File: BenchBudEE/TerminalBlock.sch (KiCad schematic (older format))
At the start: 0 parts

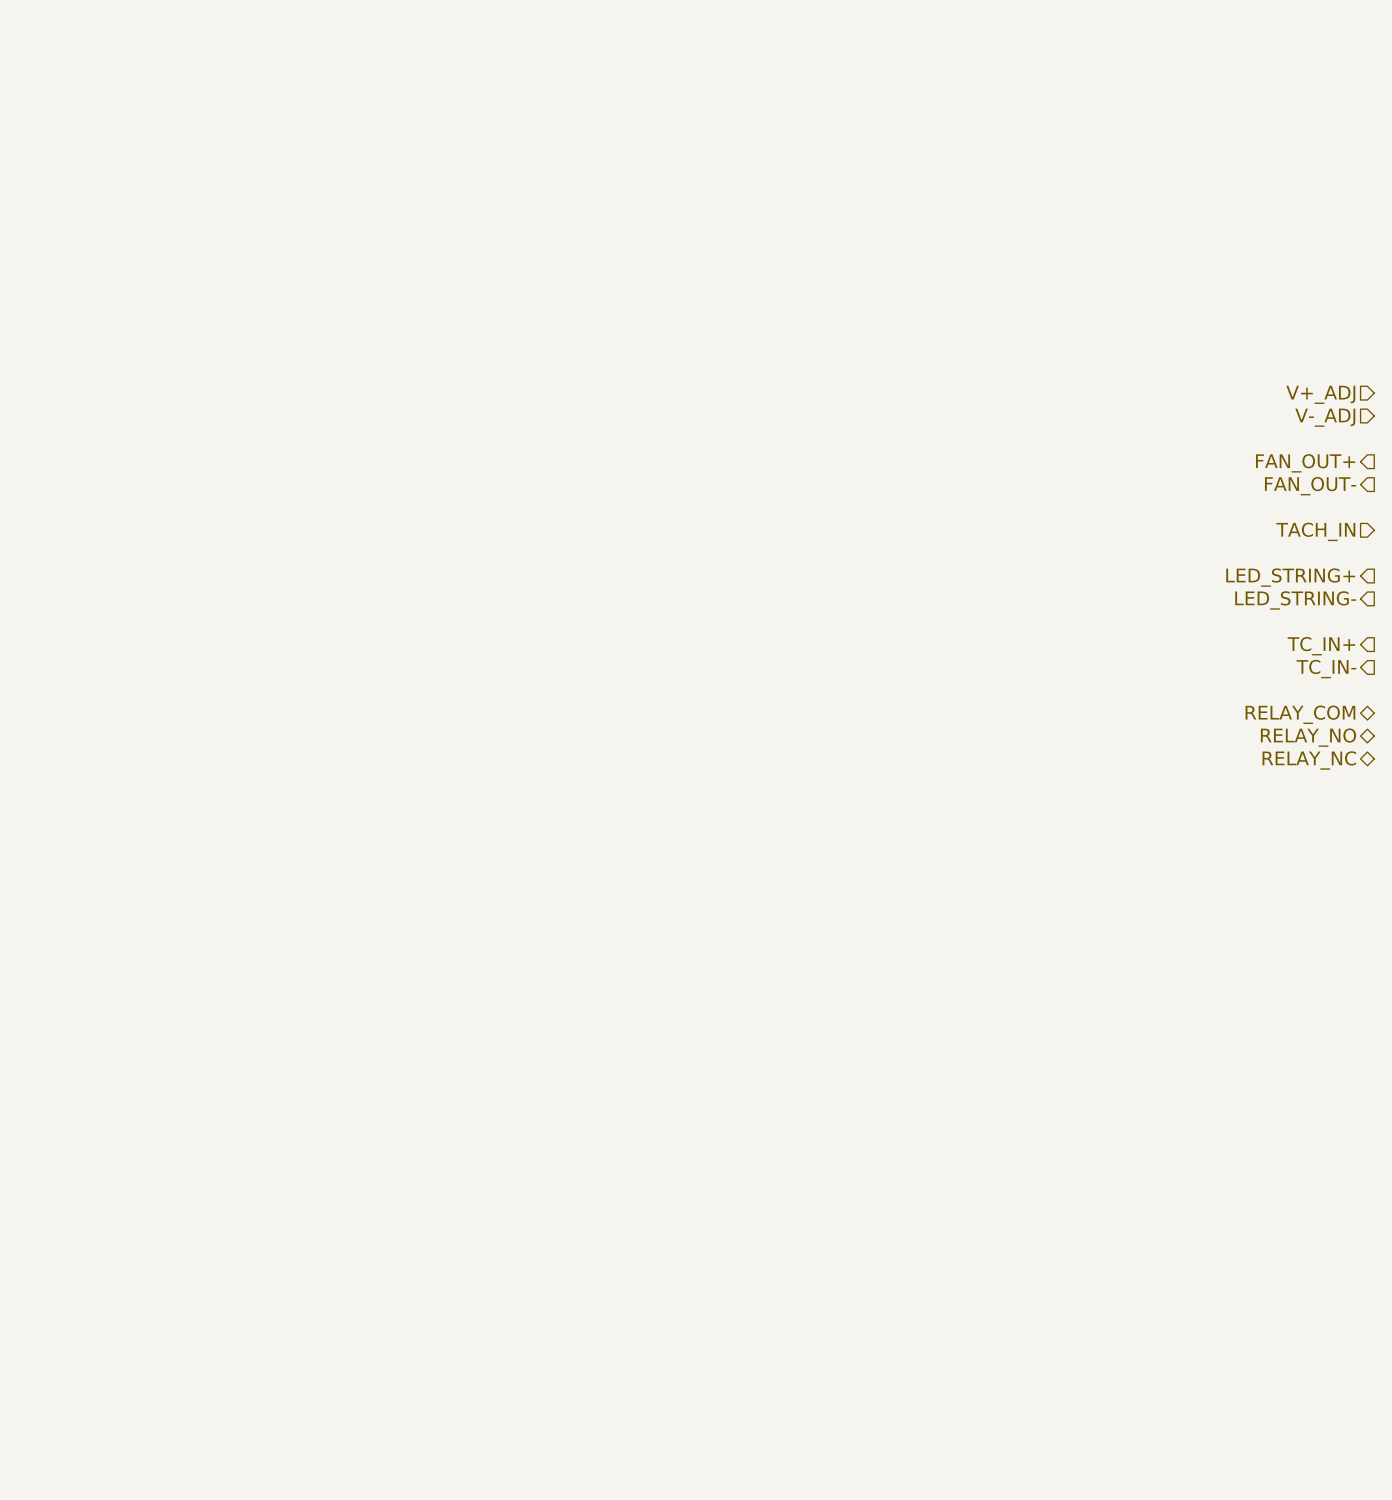
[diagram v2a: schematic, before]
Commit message: syncing to https://github.com/ContextualElectronics/BenchBudEE/tree/ebd662c68b928f78643cdf924dc35a4d91f03121
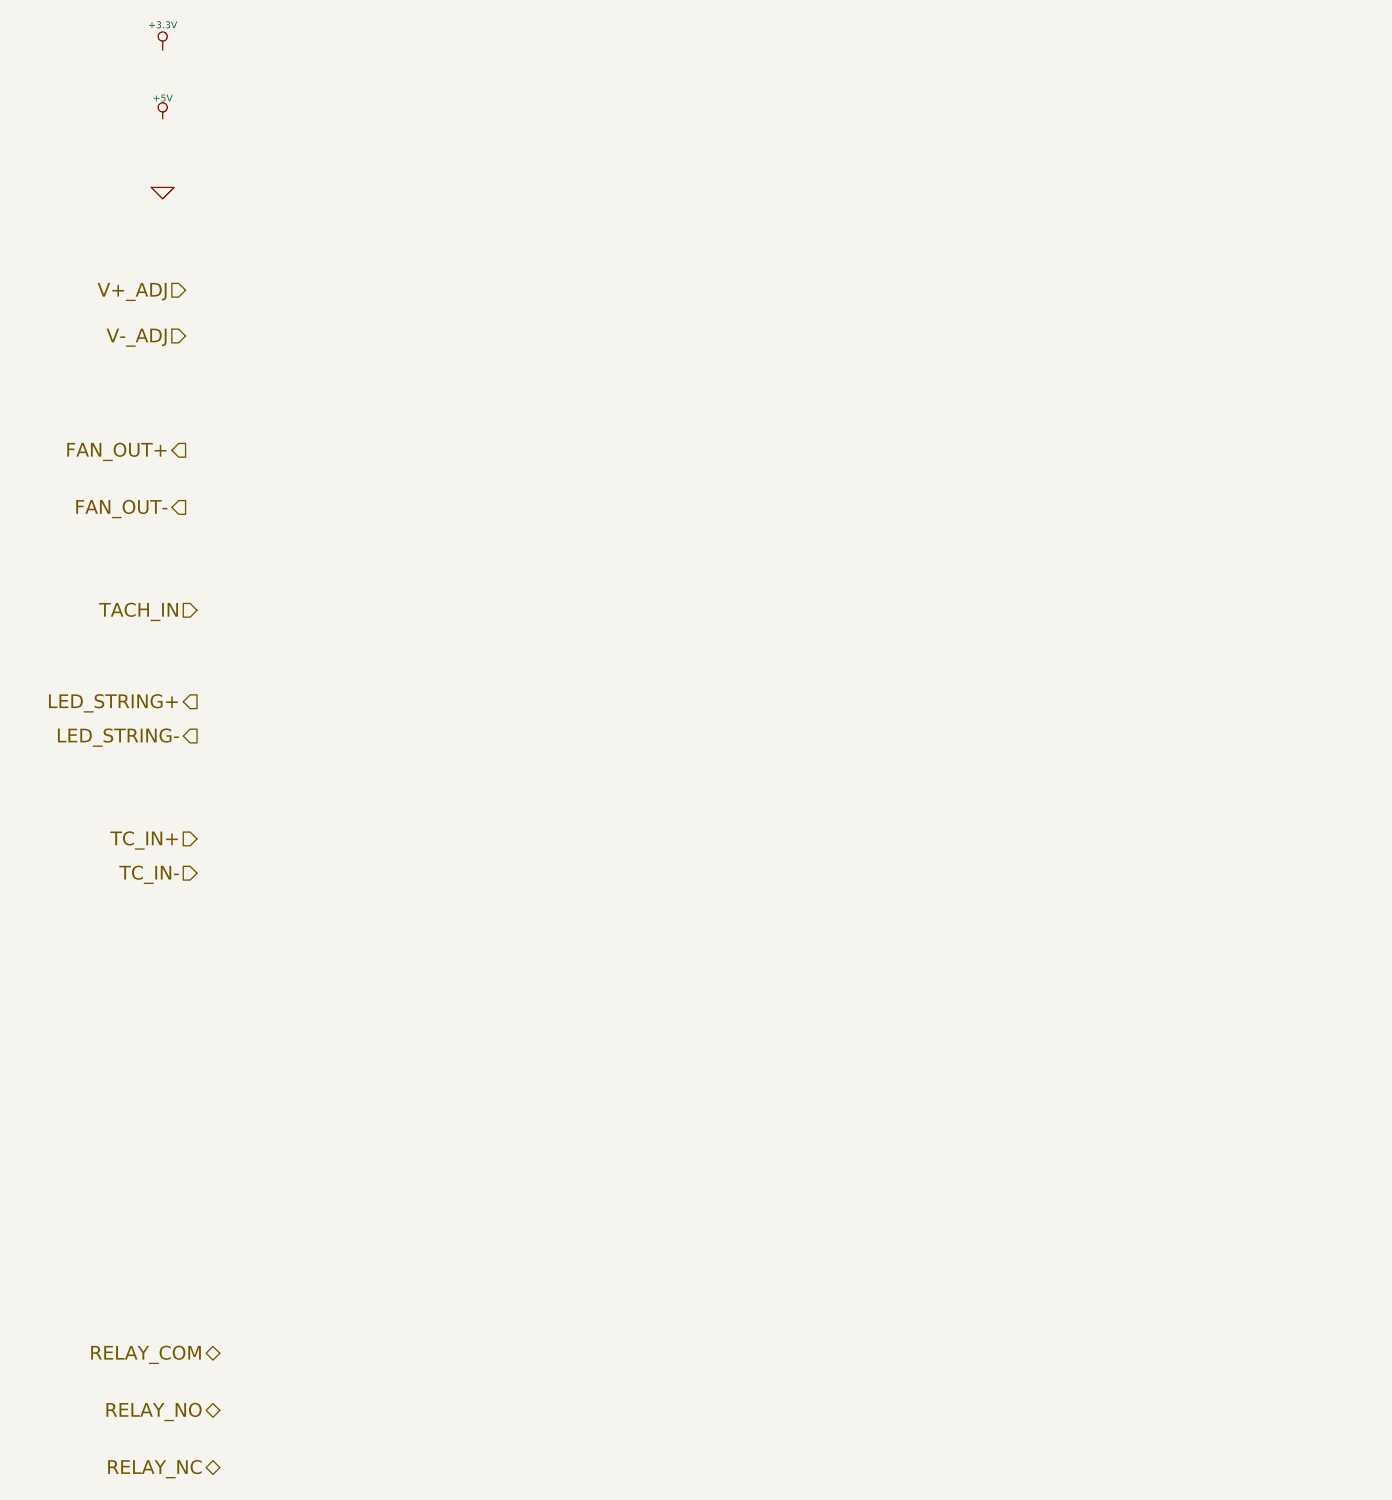
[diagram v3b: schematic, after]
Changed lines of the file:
@@
-EESchema Schematic File Version 2
+EESchema Schematic File Version 2  date 10/10/2013 12:18:22 AM
 LIBS:power
 LIBS:device
@@
 LIBS:contrib
 LIBS:valves
-LIBS:relay_spdt
-LIBS:5566-20A
-LIBS:AP5726
-LIBS:arduino
-LIBS:BenchBudEE-cache
+LIBS:BenchBuddy
+LIBS:BenchBuddy-cache
 EELAYER 27 0
 EELAYER END
 $Descr A4 11693 8268
 encoding utf-8
-Sheet 7 9
+Sheet 8 9
 Title ""
-Date "24 feb 2014"
+Date "10 oct 2013"
 Rev ""
 Comp ""
@@
 Comment4 ""
 $EndDescr
-Text HLabel 7050 2450 0    60   Input ~ 0
+Text HLabel 1850 2000 0    60   Input ~ 0
 V+_ADJ
-Text HLabel 7050 2550 0    60   Input ~ 0
+Text HLabel 1850 2200 0    60   Input ~ 0
 V-_ADJ
-Text HLabel 7050 2750 0    60   Output ~ 0
+Text HLabel 1850 2700 0    60   Output ~ 0
 FAN_OUT+
-Text HLabel 7050 2850 0    60   Output ~ 0
+Text HLabel 1850 2950 0    60   Output ~ 0
 FAN_OUT-
-Text HLabel 7050 3050 0    60   Input ~ 0
+Text HLabel 1900 3400 0    60   Input ~ 0
 TACH_IN
-Text HLabel 7050 3250 0    60   Output ~ 0
+Text HLabel 1900 3800 0    60   Output ~ 0
 LED_STRING+
-Text HLabel 7050 3350 0    60   Output ~ 0
+Text HLabel 1900 3950 0    60   Output ~ 0
 LED_STRING-
-Text HLabel 7050 3550 0    60   Output ~ 0
+Text HLabel 1900 4400 0    60   Input ~ 0
 TC_IN+
-Text HLabel 7050 3650 0    60   Output ~ 0
+Text HLabel 1900 4550 0    60   Input ~ 0
 TC_IN-
-Text HLabel 7050 3850 0    60   BiDi ~ 0
+Text HLabel 2000 6650 0    60   BiDi ~ 0
 RELAY_COM
-Text HLabel 7050 3950 0    60   BiDi ~ 0
+Text HLabel 2000 6900 0    60   BiDi ~ 0
 RELAY_NO
-Text HLabel 7050 4050 0    60   BiDi ~ 0
+Text HLabel 2000 7150 0    60   BiDi ~ 0
 RELAY_NC
+$Comp
+L +3.3V #PWR?
+U 1 1 523FFDA7
+P 1750 950
+F 0 "#PWR?" H 1750 910 30  0001 C CNN
+F 1 "+3.3V" H 1750 1060 30  0000 C CNN
+F 2 "~" H 1750 950 60  0000 C CNN
+F 3 "~" H 1750 950 60  0000 C CNN
+	1    1750 950
+	1    0    0    -1
+$EndComp
+$Comp
+L +5V #PWR?
+U 1 1 523FFDB6
+P 1750 1250
+F 0 "#PWR?" H 1750 1340 20  0001 C CNN
+F 1 "+5V" H 1750 1340 30  0000 C CNN
+F 2 "~" H 1750 1250 60  0000 C CNN
+F 3 "~" H 1750 1250 60  0000 C CNN
+	1    1750 1250
+	1    0    0    -1
+$EndComp
+$Comp
+L GND #PWR?
+U 1 1 523FFDC5
+P 1750 1550
+F 0 "#PWR?" H 1750 1550 30  0001 C CNN
+F 1 "GND" H 1750 1480 30  0001 C CNN
+F 2 "~" H 1750 1550 60  0000 C CNN
+F 3 "~" H 1750 1550 60  0000 C CNN
+	1    1750 1550
+	1    0    0    -1
+$EndComp
 $EndSCHEMATC
